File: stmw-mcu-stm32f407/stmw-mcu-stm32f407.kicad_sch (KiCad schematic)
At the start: 40 parts, among them J2 TYPE-C-31-M-12, SW1 TS-1088R-02526, SW2 TS-1088R-02526, U1 AMS1117-3.3, U3 STM32F407VETx, Y1 X_16MHZ

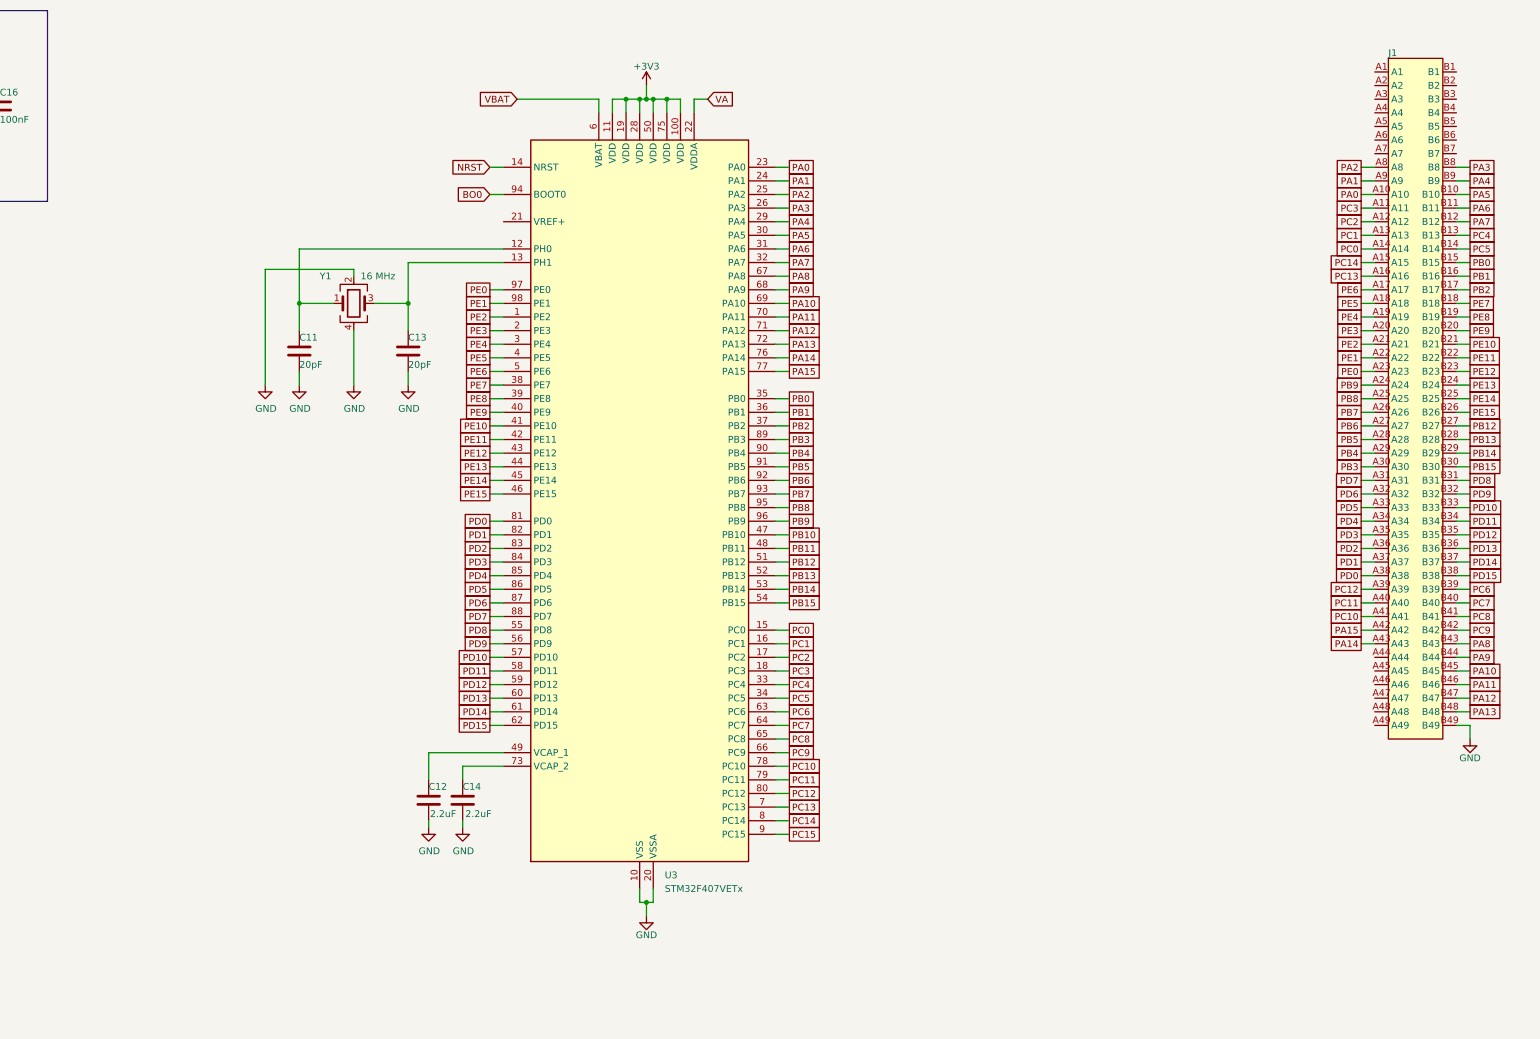
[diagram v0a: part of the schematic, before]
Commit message: Hmmmm
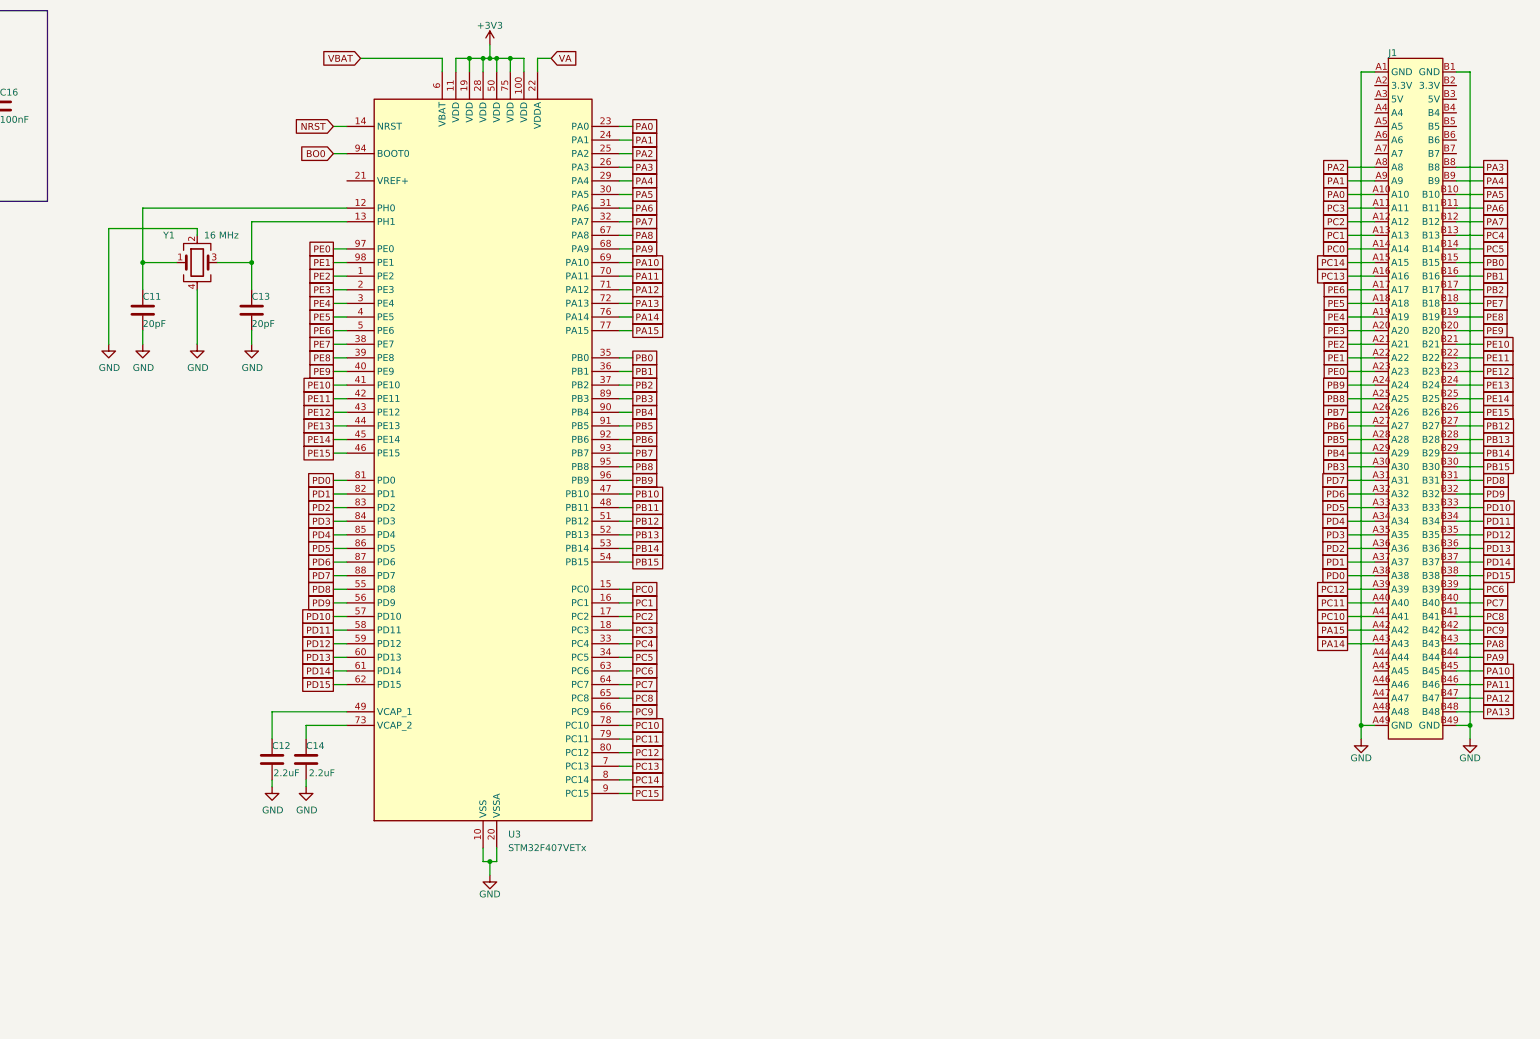
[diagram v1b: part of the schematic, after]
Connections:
- net GND: now also J1.A1 (GND), J1.A49 (GND), J1.B1 (GND)
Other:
- moved on the sheet: C11, C12, C13, C14, U3, Y1
